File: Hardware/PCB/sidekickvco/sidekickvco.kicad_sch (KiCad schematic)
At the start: 17 parts, among them J1 Conn_01x06, J10 Conn_01x03, J11 Conn_01x04, J12 3_pin_Molex_connector, J13 Wire pads, J14 Conn_01x01, J15 Conn_01x01, J16 Conn_01x01, J17 Conn_02x04_Odd_Even, J2 Conn_01x03, J3 Conn_01x04, J4 3_pin_Molex_header, J5 Wire pads, J6 Conn_01x01, J7 Conn_01x01, J8 Conn_01x01, J9 Conn_01x06

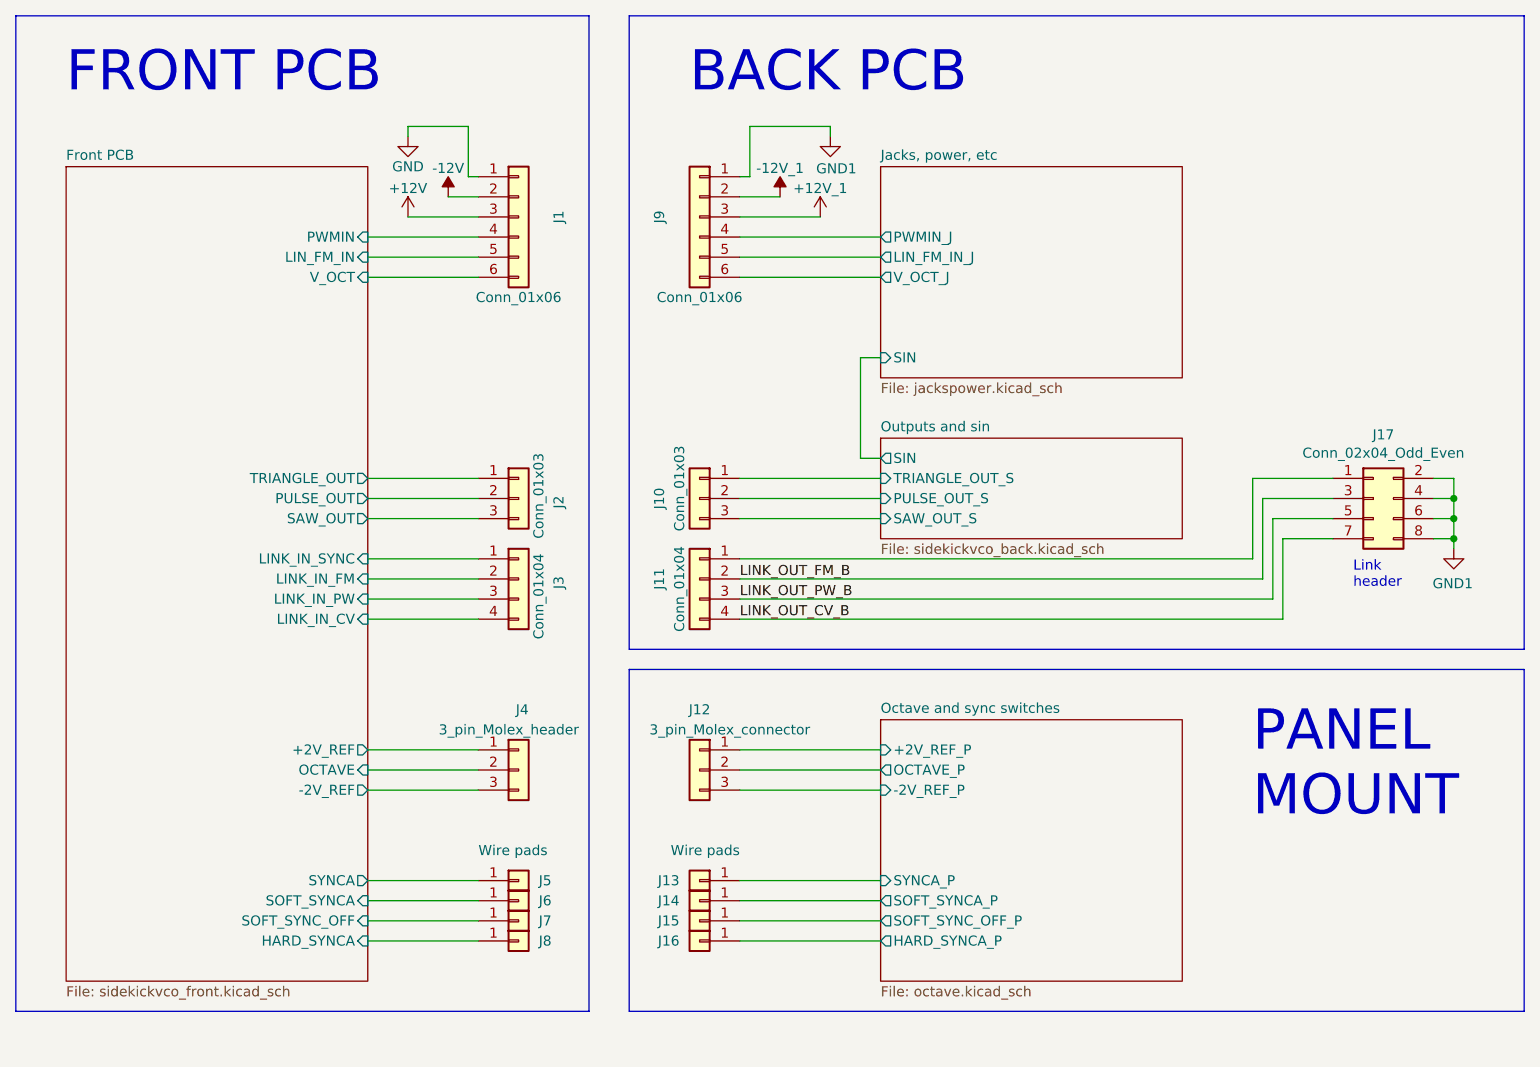
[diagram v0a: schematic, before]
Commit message: Initial version of circuit and layout
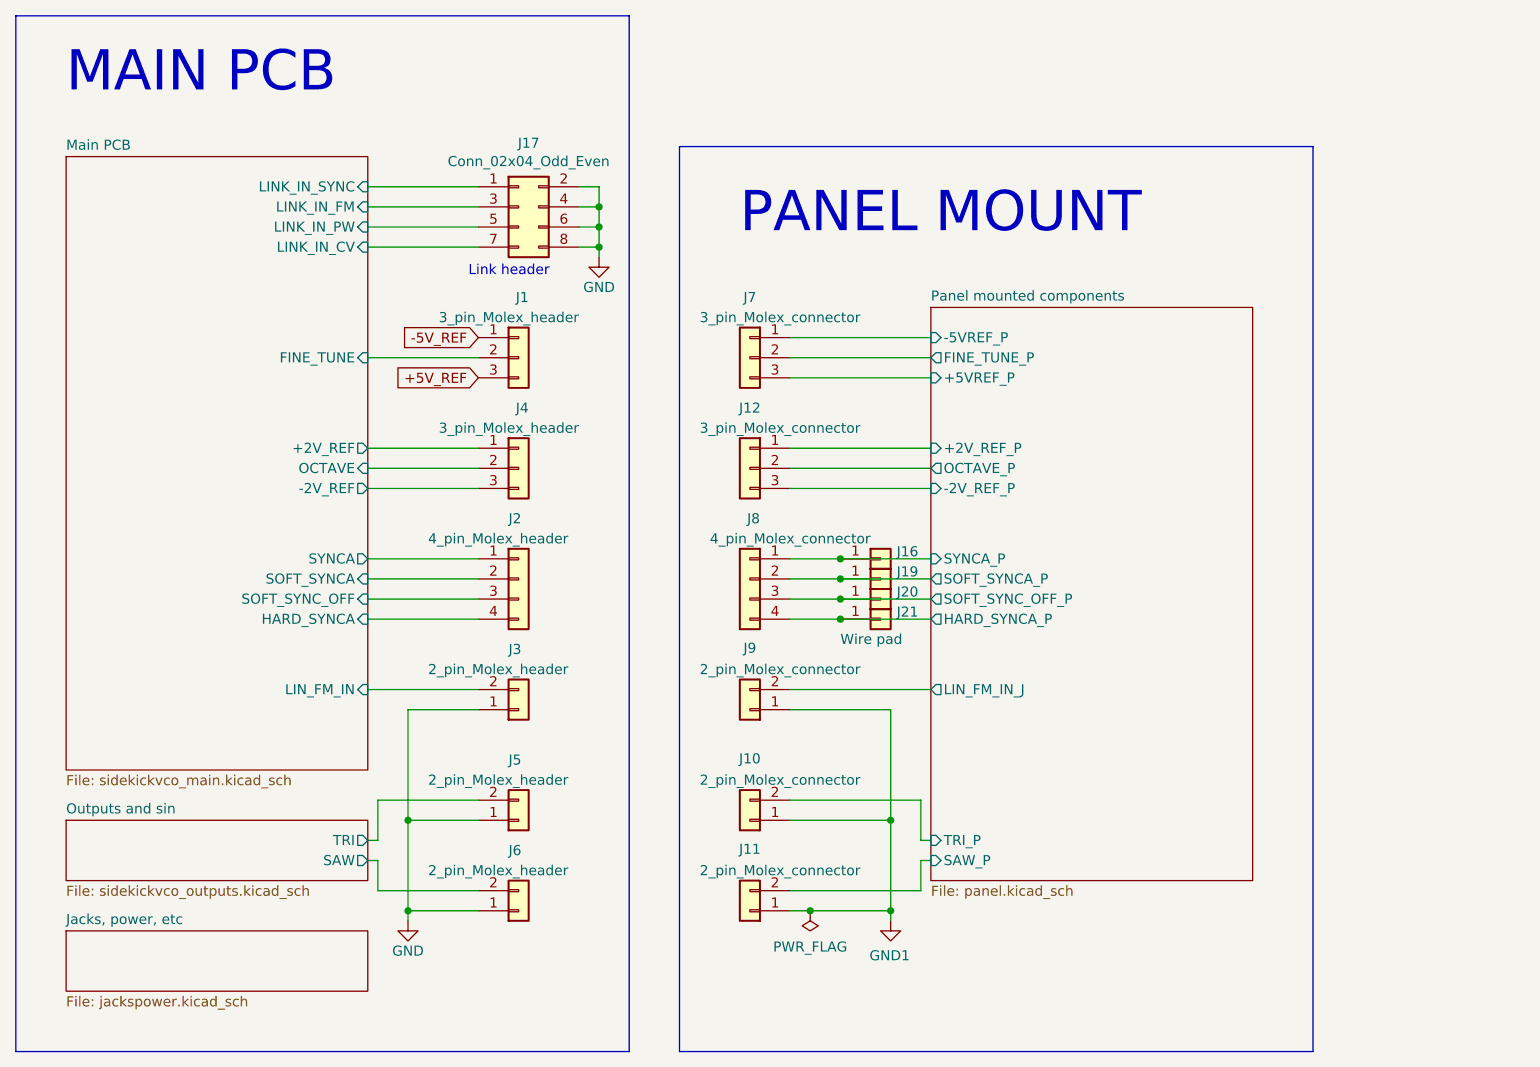
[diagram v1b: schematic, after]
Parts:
- removed J1: Conn_01x06, Connector_PinHeader_2.54mm:PinHeader_1x06_P2.54mm_Vertical, symbol Connector_Generic:Conn_01x06
- removed J10: Conn_01x03, Connector_PinSocket_2.54mm:PinSocket_1x03_P2.54mm_Vertical, symbol Connector_Generic:Conn_01x03
- removed J11: Conn_01x04, Connector_PinSocket_2.54mm:PinSocket_1x04_P2.54mm_Vertical, symbol Connector_Generic:Conn_01x04
- removed J13, J5: Wire pads, Connector_Wire:SolderWire-0.5sqmm_1x01_D0.9mm_OD2.1mm, symbol Connector_Generic:Conn_01x01
- removed J14, J15, J6, J7, J8: Conn_01x01, herovco:SolderWire-round_1x01_D0.9mm_OD2.1mm, symbol Connector_Generic:Conn_01x01
- removed J2: Conn_01x03, Connector_PinHeader_2.54mm:PinHeader_1x03_P2.54mm_Vertical, symbol Connector_Generic:Conn_01x03
- removed J3: Conn_01x04, Connector_PinHeader_2.54mm:PinHeader_1x04_P2.54mm_Vertical, symbol Connector_Generic:Conn_01x04
- removed J9: Conn_01x06, Connector_PinSocket_2.54mm:PinSocket_1x06_P2.54mm_Vertical, symbol Connector_Generic:Conn_01x06
- added J1: 3_pin_Molex_header, ao_tht:Molex_KK-254_AE-6410-03A_1x03_P2.54mm_Vertical, symbol ao_symbols:3_pin_Molex_header
- added J10, J11, J9: 2_pin_Molex_connector, symbol ao_symbols:2_pin_Molex_connector
- added J19, J20, J21: Wire pad, Connector_Wire:SolderWire-0.5sqmm_1x01_D0.9mm_OD2.1mm, symbol Connector_Generic:Conn_01x01
- added J2: 4_pin_Molex_header, Connector_Molex:Molex_KK-254_AE-6410-04A_1x04_P2.54mm_Vertical, symbol Connector_Generic:Conn_01x04
- added J3, J5, J6: 2_pin_Molex_header, ao_tht:Molex_KK-254_AE-6410-02A_1x02_P2.54mm_Vertical, symbol ao_symbols:2_pin_Molex_header
- added J7: 3_pin_Molex_connector, ao_tht:Molex_KK-254_AE-6410-03A_1x03_P2.54mm_Vertical, symbol ao_symbols:3_pin_Molex_connector
- added J8: 4_pin_Molex_connector, symbol Connector_Generic:Conn_01x04
- J16: value Conn_01x01 -> Wire pad; footprint herovco:SolderWire-round_1x01_D0.9mm_OD2.1mm -> Connector_Wire:SolderWire-0.5sqmm_1x01_D0.9mm_OD2.1mm
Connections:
- net LINK_OUT_CV_B is gone; now on net Main PCB/LINK_IN_CV: J17.7 (Pin_7)
- net LINK_OUT_FM_B is gone; now on net Main PCB/LINK_IN_FM: J17.3 (Pin_3)
- net LINK_OUT_PW_B is gone; now on net Main PCB/LINK_IN_PW: J17.5 (Pin_5)
- net Main PCB/HARD_SYNCA: now also J2.4 (Pin_4)
- net Main PCB/LINK_IN_SYNC: now also J17.1 (Pin_1)
- net Main PCB/LIN_FM_IN: now also J3.2 (Pin_2)
- net Main PCB/SOFT_SYNCA: now also J2.2 (Pin_2)
- net Main PCB/SOFT_SYNC_OFF: now also J2.3 (Pin_3)
- net Main PCB/SYNCA: now also J2.1 (Pin_1)
- net GND: now also J17.2 (Pin_2), J17.4 (Pin_4), J17.6 (Pin_6), J17.8 (Pin_8), J3.1 (Pin_1), J5.1 (Pin_1), J6.1 (Pin_1)
- net GND1: now also J10.1 (Pin_1), J11.1 (Pin_1), J9.1 (Pin_1); no longer J17.2 (Pin_2), J17.4 (Pin_4), J17.6 (Pin_6), J17.8 (Pin_8)
- net Panel mounted components/HARD_SYNCA_P: now also J21.1 (Pin_1), J8.4 (Pin_4); no longer J16.1 (Pin_1)
- net Panel mounted components/SOFT_SYNCA_P: now also J19.1 (Pin_1), J8.2 (Pin_2)
- net Panel mounted components/SOFT_SYNC_OFF_P: now also J20.1 (Pin_1), J8.3 (Pin_3)
- net Panel mounted components/SYNCA_P: now also J16.1 (Pin_1), J8.1 (Pin_1)
- new net +5V_REF: J1.3 (Pin_3)
- new net -5V_REF: J1.1 (Pin_1)
- new net Main PCB/FINE_TUNE: J1.2 (Pin_2)
- new net Outputs and sin/SAW: J6.2 (Pin_2)
- new net Outputs and sin/TRI: J5.2 (Pin_2)
- new net Panel mounted components/+5VREF_P: J7.3 (Pin_3)
- new net Panel mounted components/-5VREF_P: J7.1 (Pin_1)
- new net Panel mounted components/FINE_TUNE_P: J7.2 (Pin_2)
- new net Panel mounted components/LIN_FM_IN_J: J9.2 (Pin_2)
- new net Panel mounted components/SAW_P: J11.2 (Pin_2)
- new net Panel mounted components/TRI_P: J10.2 (Pin_2)
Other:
- sheet Front PCB renamed Main PCB
- sheet Octave and sync switches renamed Panel mounted components
- sheet Jacks, power, etc ports: added none; removed LIN_FM_IN_J, PWMIN_J, SIN, V_OCT_J
- sheet Main PCB: file sidekickvco_front.kicad_sch -> sidekickvco_main.kicad_sch
- sheet Main PCB ports: added FINE_TUNE; removed PULSE_OUT, PWMIN, SAW_OUT, TRIANGLE_OUT, V_OCT
- sheet Outputs and sin: file sidekickvco_back.kicad_sch -> sidekickvco_outputs.kicad_sch
- sheet Outputs and sin ports: added SAW, TRI; removed PULSE_OUT_S, SAW_OUT_S, SIN, TRIANGLE_OUT_S
- sheet Panel mounted components: file octave.kicad_sch -> panel.kicad_sch
- sheet Panel mounted components ports: added +5VREF_P, -5VREF_P, FINE_TUNE_P, LIN_FM_IN_J, SAW_P, TRI_P; removed none
- note added: "MAIN PCB"
- note removed: "BACK PCB"
- note removed: "FRONT PCB"
- moved on the sheet: J12, J17, J4
